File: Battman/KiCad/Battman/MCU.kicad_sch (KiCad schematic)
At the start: 53 parts, among them IC700 STM32L552RET6, IC701 ISO1044BDR, IC702 ESDA6V1-5SC6, J700 FTSH-105-01-L-DV-K, Y700 FC-135_32.7680KA-AG0

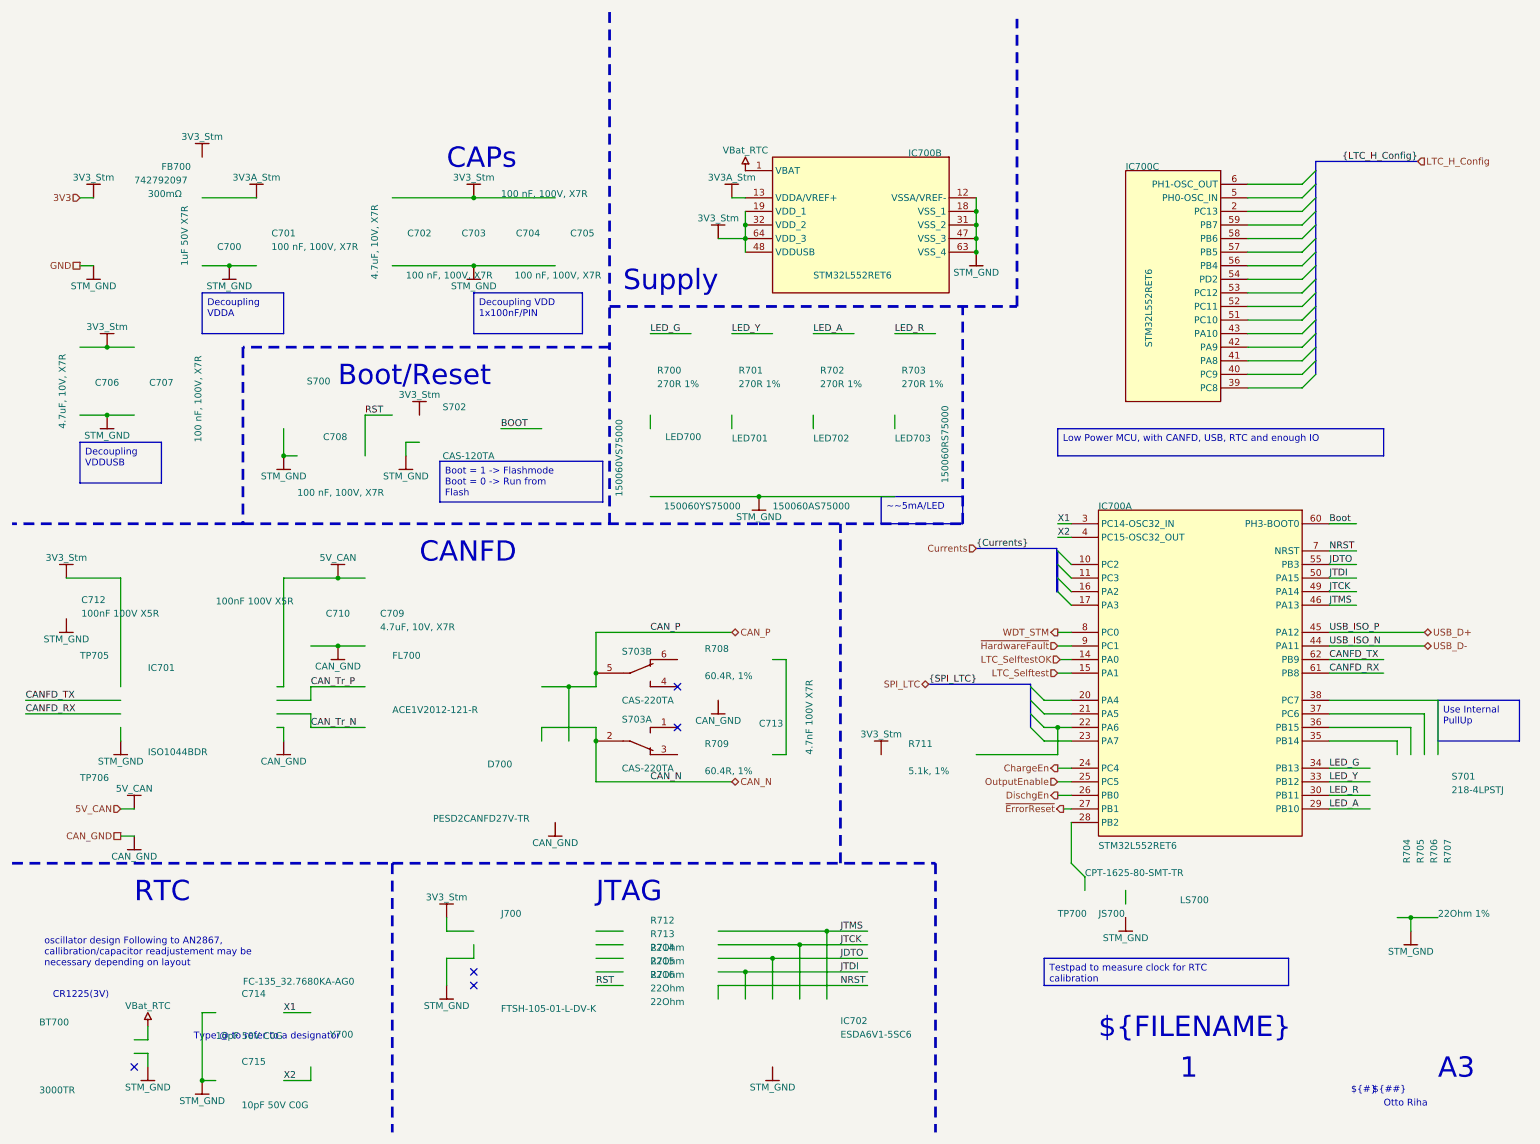
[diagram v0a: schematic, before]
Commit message: kicad release
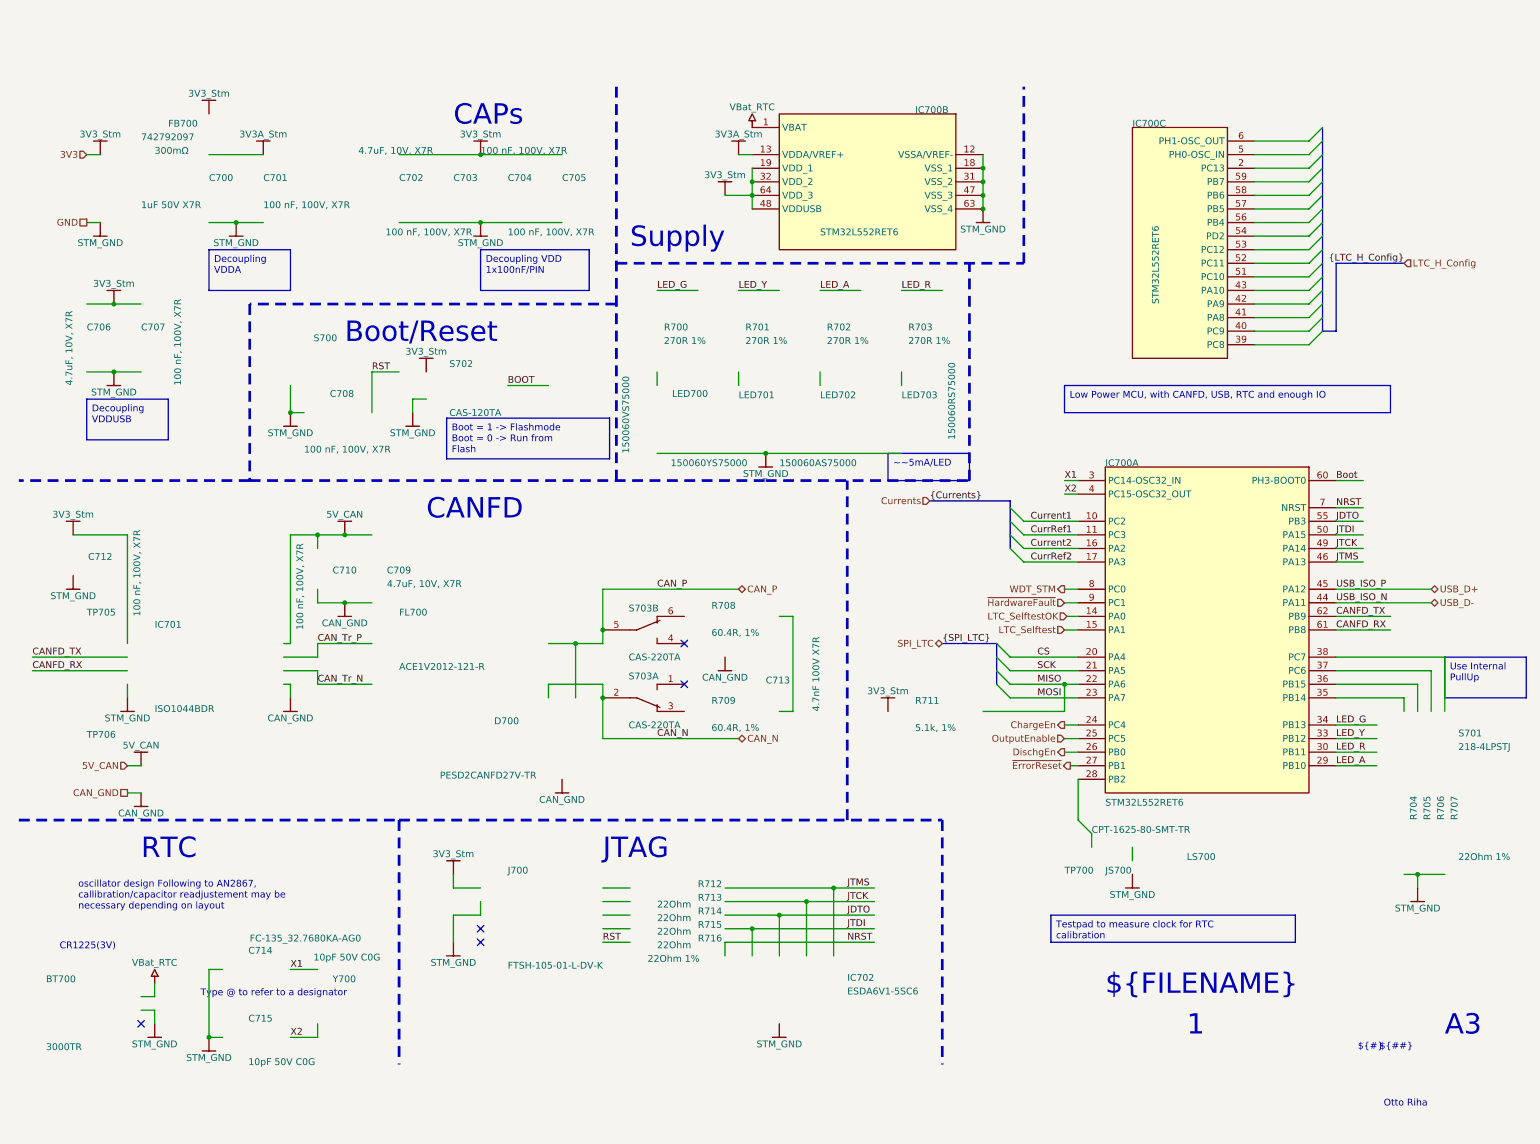
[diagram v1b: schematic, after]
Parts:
- removed C710: 100nF 100V X5R, C__Users_otto_Documents_AltiumLL_SamacSys.PcbLib:CAPC1608X90N, symbol Battman-altium-import:MCU_1_mirrored_HMK107BJ104KA-T_SamacSys.SchLib
- removed C712: 100nF 100V X5R, C__Users_otto_Documents_AltiumLL_SamacSys.PcbLib:CAPC1608X90N, symbol Battman-altium-import:MCU_1_HMK107BJ104KA-T_SamacSys.SchLib
- added C710, C712: 100 nF, 100V, X7R, C__Users_otto_Documents_AltiumLL_SamacSys.PcbLib:MAJx16, symbol Battman-altium-import:MCU_1_MAJCH168BB7104KTEA01_SamacSys.SchLib
- R707: ALTIUM_VALUE 22Ohm 1% -> 22Ohm
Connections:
- net Current1: now reaches IC700.10 (PC2)
- net CurrRef1: now reaches IC700.11 (PC3)
- net Current2: now reaches IC700.16 (PA2)
- net CurrRef2: now reaches IC700.17 (PA3)
- net CS: now reaches IC700.20 (PA4)
- net SCK: now reaches IC700.21 (PA5)
- net MISO: now reaches IC700.22 (PA6)
- net MOSI: now reaches IC700.23 (PA7)
